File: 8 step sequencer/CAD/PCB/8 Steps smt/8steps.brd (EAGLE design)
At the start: 105.4 x 36.5 mm, 30 parts, among them IC1 4040N, IC2 4040N, IC3 7805TV, IC4 4051N, IC5 4051N, IC6 LM324N

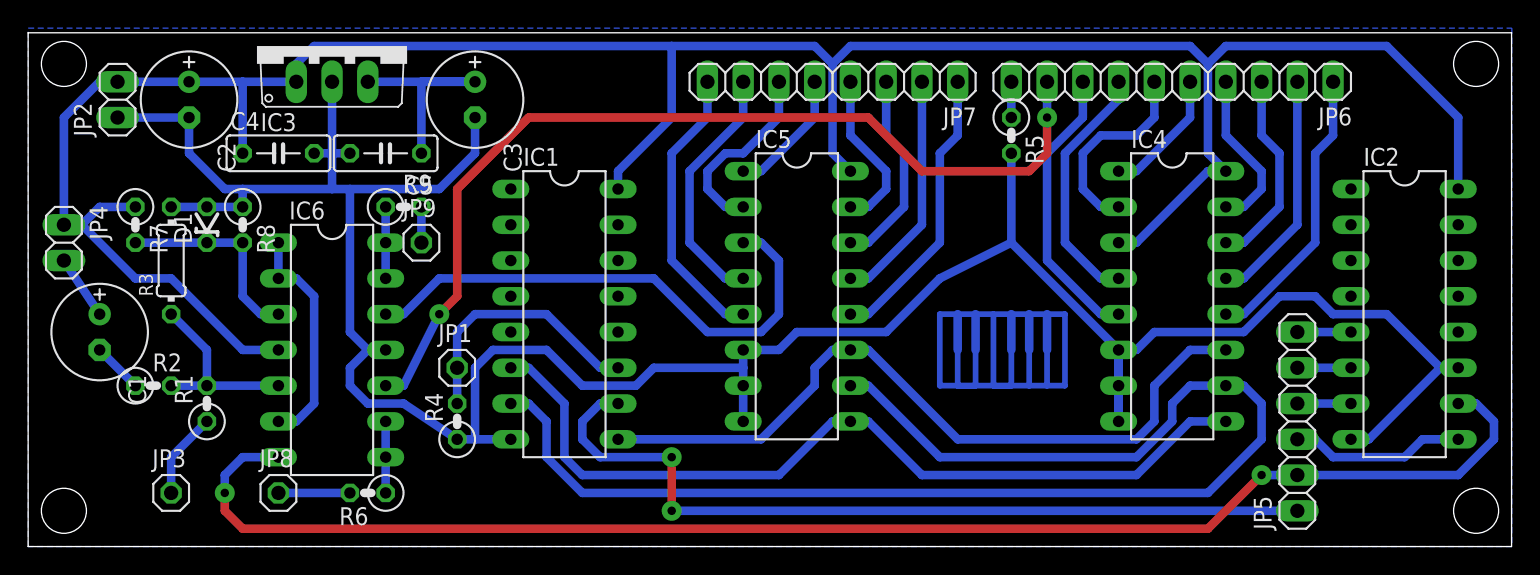
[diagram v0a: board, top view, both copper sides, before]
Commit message: new fabrication files of  8 steps
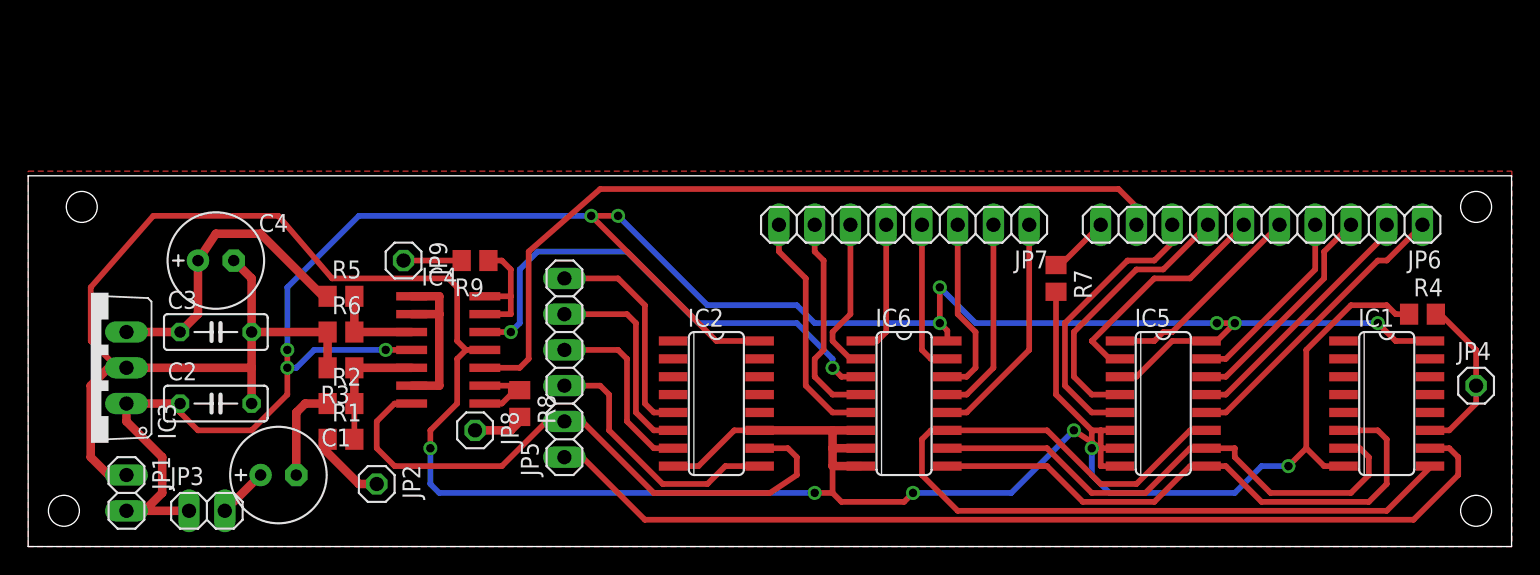
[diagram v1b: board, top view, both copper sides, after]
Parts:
- removed C5: 100n, rcl:C050-025X075
- removed D1: 2.5v, diode:ZDIO-2.5
- C2: value 100u -> 100n; device rcl:E2,5-7 -> rcl:C050-025X075
- C3: value 47u -> 100n; device rcl:E2,5-7 -> rcl:C050-025X075
- C4: value 100n -> 47u; device rcl:C050-025X075 -> rcl:E2,5-7
- IC1, IC2: value 4040N -> 4040D; device 40xx:DIL16 -> 40xx:SO16
- IC4: value 4051N -> TL084D; device 40xx:DIL16 -> linear:SO14
- IC5: value 4051N -> 4051D; device 40xx:DIL16 -> 40xx:SO16
- IC6: value LM324N -> 4051D; device linear:DIL14 -> 40xx:SO16
- JP1: value RST -> PWR; device pinhead:1X01 -> pinhead:1X02
- JP2: value PWR -> CK_IN; device pinhead:1X02 -> pinhead:1X01
- JP3: value CK_IN -> TRG; device pinhead:1X01 -> pinhead:1X02
- JP4: value TRG -> RST; device pinhead:1X02 -> pinhead:1X01
- JP6: value (none) -> GATE/LED
- JP7: value (none) -> POT
- R1, R2, R9: device rcl:0207/2V -> rcl:R0805
- R3: device rcl:0204/7 -> rcl:R0805
- R4: value 100k -> 10k; device rcl:0207/2V -> rcl:R0805
- R5: value 100k -> 1k; device rcl:0207/2V -> rcl:R0805
- R6: value 1K -> 1k; device rcl:0207/2V -> rcl:R0805
- R7: value 330 -> 100k; device rcl:0207/2V -> rcl:R0805
- R8: value Rz -> 1K; device rcl:0207/2V -> rcl:R0805
- moved JP4 100.8 mm to (102.9, 11.4), turned to 0 degrees
- moved R4 69.0 mm to (99.1, 16.5), turned to 0 degrees
- moved R7 65.5 mm to (73.0, 19.1)
- moved IC1 58.8 mm to (96.5, 10.2)
- moved JP5 52.2 mm to (38.1, 12.7)
- moved IC4 51.6 mm to (29.8, 14.0)
- moved IC2 49.3 mm to (48.9, 10.2)
- moved R5 49.0 mm to (22.2, 17.8), turned to 0 degrees
- moved IC6 40.8 mm to (62.2, 10.2)
- moved JP2 32.9 mm to (24.8, 4.45), turned to 270 degrees
- moved IC3 28.6 mm to (4.45, 12.7), turned to 90 degrees
- moved IC5 27.1 mm to (80.6, 10.2)
- moved JP1 25.1 mm to (6.99, 3.81), turned to 270 degrees
- moved C3 24.7 mm to (13.3, 15.2), turned to 0 degrees
- moved R8 23.4 mm to (34.9, 10.2)
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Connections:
- net B0: now also IC6.11; no longer IC4.11
- net B1: now also IC6.10; no longer IC4.10
- net B2: now also IC6.9; no longer IC4.9
- net GATE_RAW: now also IC4.10; no longer IC6.10
- net GND: now also C2.2, C3.2, C4.-, IC4.11, IC6.6, IC6.7, IC6.8, JP1.1, R6.1, R7.2; no longer C2.-, C3.-, C4.2, C5.2, D1.A, IC4.6, IC4.7, IC4.8, IC6.11, JP2.1, R5.2, R8.1
- net N$1: now also IC4.3, R5.2, R6.2; no longer D1.C, IC6.3, R7.2, R8.2
- net N$10: now also IC5.12; no longer IC4.12
- net N$11: now also IC5.13; no longer IC4.13
- net N$12: now also IC5.14; no longer IC4.14
- net N$13: now also IC5.15; no longer IC4.15
- net N$14: now also IC5.1; no longer IC4.1
- net N$15: now also IC5.4; no longer IC4.4
- net N$16: now also IC5.2; no longer IC4.2
- net N$17: now also IC5.5; no longer IC4.5
- net N$18: now also IC6.12; no longer IC5.12
- net N$19: now also IC6.13; no longer IC5.13
- net N$20: now also IC6.14; no longer IC5.14
- net N$21: now also IC6.15; no longer IC5.15
- net N$22: now also IC6.1; no longer IC5.1
- net N$23: now also IC6.4; no longer IC5.4
- net N$25: now also IC6.5; no longer IC5.5
- net N$26: now also IC4.13, IC4.14; no longer IC6.13, IC6.14
- net N$28: now also R7.1; no longer R5.1
- net N$29: now also JP4.1; no longer JP1.1
- net N$3: now also IC4.12, IC6.3; no longer IC5.3, IC6.12
- net N$30: now also IC4.8, IC4.9, R8.1; no longer IC6.8, IC6.9, R6.1
- net N$31: now also R8.2; no longer R6.2
- net N$32: now also IC6.2; no longer IC5.2
- net N$33: now also IC4.5; no longer IC6.5
- net N$34: now also JP3.2; no longer JP4.2
- net N$35: now also JP2.1; no longer JP3.1
- net N$4: now also IC4.7; no longer IC6.7
- net V5V: now also C3.1, C4.+, R5.1; no longer C3.+, C5.1
- net VCC: now also C2.1, IC4.4, IC5.3, IC6.16, JP1.2, JP3.1; no longer C2.+, C4.1, IC4.16, IC4.3, IC6.4, JP2.2, JP4.1, R7.1
- net V_REF: now also IC4.1, IC4.2, IC4.6; no longer IC6.1, IC6.2, IC6.6
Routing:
- net N$24: track 73.7 -> 0.00 mm
- net N$4: track 104.5 -> 43.3 mm, vias 2 -> 0
- net B1: track 96.3 -> 38.1 mm
- net GND: track 194.7 -> 223.5 mm, vias 0 -> 6
- net VCC: track 184.9 -> 161.7 mm, vias 0 -> 10
- net B2: track 60.9 -> 41.4 mm
- net N$8: track 3.81 -> 15.8 mm
- net B0: track 53.3 -> 64.7 mm
- net N$7: track 3.81 -> 14.9 mm
- net N$9: track 59.5 -> 70.2 mm, vias 2 -> 0
- net GATE_RAW: track 67.6 -> 57.6 mm, vias 2 -> 0
- net N$6: track 3.81 -> 13.2 mm
- net N$1: track 14.5 -> 6.61 mm
- net N$29: track 18.6 -> 11.8 mm
- net N$5: track 12.5 -> 18.8 mm
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- added copper zone on layer 1, net GND
- removed copper zone on layer 16, net GND
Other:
- board size 105.4 x 36.5 mm -> 105.4 x 26.3 mm
